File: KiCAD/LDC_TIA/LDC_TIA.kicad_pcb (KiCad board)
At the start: 2 copper layers, 55.7 x 32.2 mm, 23 parts, among them J1 54-00166, J2 Conn_01x07_Pin, J3 Conn_01x02_Pin, Q1 BC817, SW1 B3F-6020, U1 OPA2197xD, U2 LTC1044, U3 LM7805_TO220

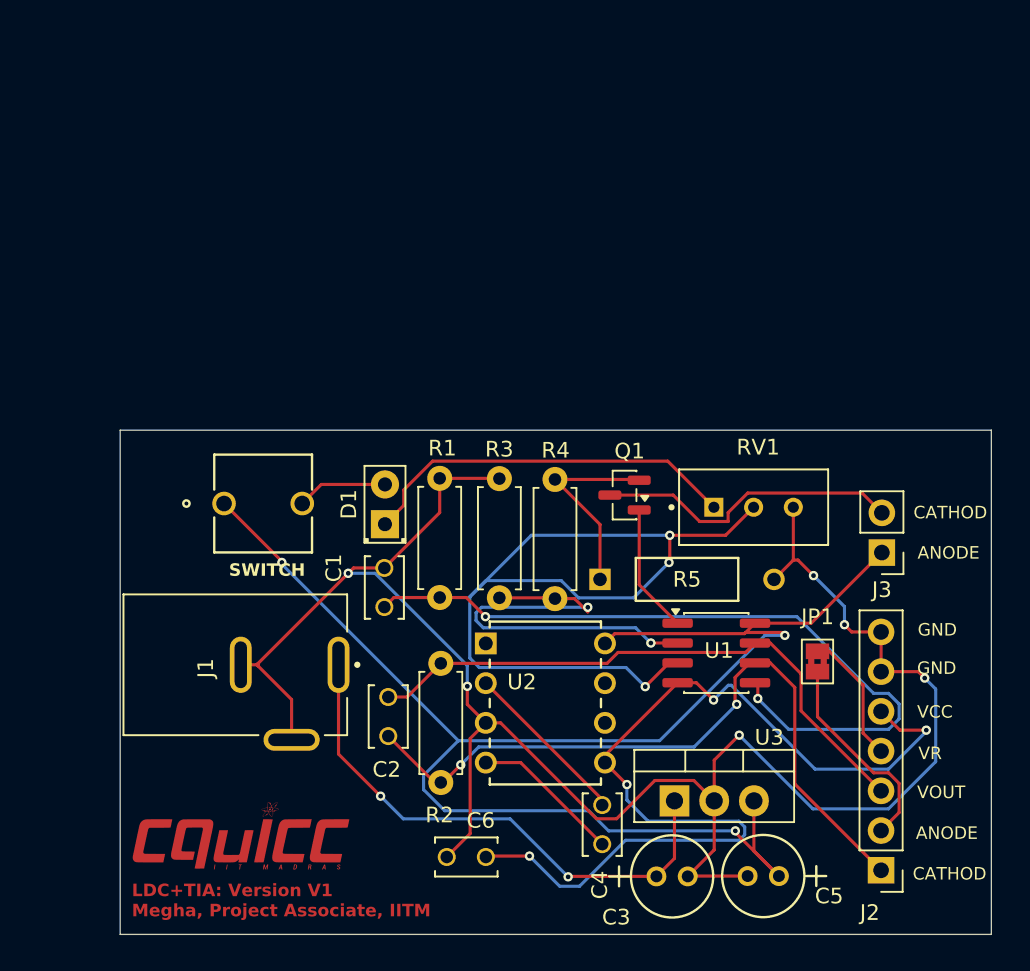
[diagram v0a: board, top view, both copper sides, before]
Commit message: PCB VOL 2
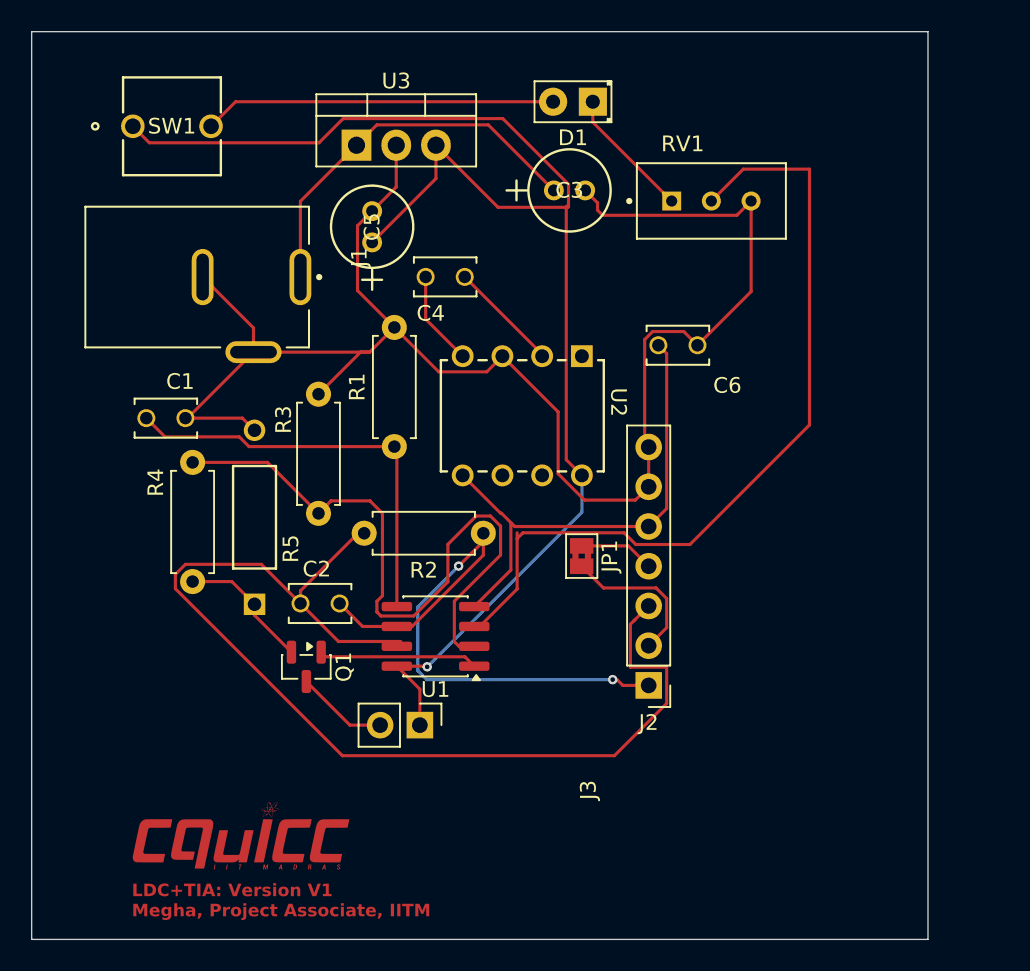
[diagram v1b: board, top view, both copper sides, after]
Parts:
- moved C5 48.1 mm to (130.8, 70.2), turned to 90 degrees
- moved U3 46.6 mm to (129.8, 63.9)
- moved C3 44.3 mm to (142.4, 66.8)
- moved C4 36.4 mm to (135.4, 72.4), turned to 180 degrees
- moved C6 35.4 mm to (150.3, 76.7), turned to 180 degrees
- moved J3 31.5 mm to (133.8, 101.0), turned to -90 degrees
- moved D1 30.1 mm to (144.9, 61.2), turned to 180 degrees
- moved J1 24.9 mm to (119.9, 72.4)
- moved SW1 24.8 mm to (115.5, 62.7)
- moved R4 24.8 mm to (119.3, 84.2), turned to -90 degrees
- moved Q1 23.1 mm to (126.6, 97.3), turned to -90 degrees
- moved R5 22.1 mm to (123.3, 93.3), turned to 90 degrees
- moved RV1 19.8 mm to (152.5, 67.5)
- moved U2 19.4 mm to (144.2, 77.4), turned to -90 degrees
- moved J2 19.0 mm to (148.5, 98.5)
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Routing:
- net /VOUT: track 38.2 -> 70.4 mm
- net /-VCC: track 60.9 -> 31.9 mm, vias 4 -> 0
- net Net-(U1B-+): track 48.1 -> 26.9 mm, vias 2 -> 0
- net GND: track 124.9 -> 105.1 mm, vias 6 -> 0
- net Net-(D1-A): track 5.80 -> 22.5 mm
- net Net-(D1-K): track 24.5 -> 8.44 mm
- net Net-(U1A--): track 28.0 -> 42.9 mm, vias 2 -> 0
- net Net-(J3-Pin_2): track 19.7 -> 5.88 mm
- net /+VCC: track 102.3 -> 91.3 mm, vias 3 -> 1
- net /VI: track 34.6 -> 24.8 mm, vias 2 -> 0
- net /CATHODE: track 46.2 -> 38.8 mm
- net Net-(Q1-E): track 13.5 -> 8.60 mm
- net Net-(U2-CAP+): track 10.9 -> 7.12 mm
- net /VR: track 8.50 -> 4.82 mm
- net /ANODE: track 13.4 -> 9.78 mm
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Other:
- board size 55.7 x 32.2 mm -> 57.3 x 58 mm
- board text removed: "ANODE"
- board text removed: "CATHOD"
- board text removed: "GND"
- board text removed: "SWITCH"
- board text removed: "VCC"
- board text removed: "VOUT"
- board text removed: "VR"
